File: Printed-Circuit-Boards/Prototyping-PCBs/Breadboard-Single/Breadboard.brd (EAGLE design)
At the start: 91.4 x 48.3 mm, 98 parts

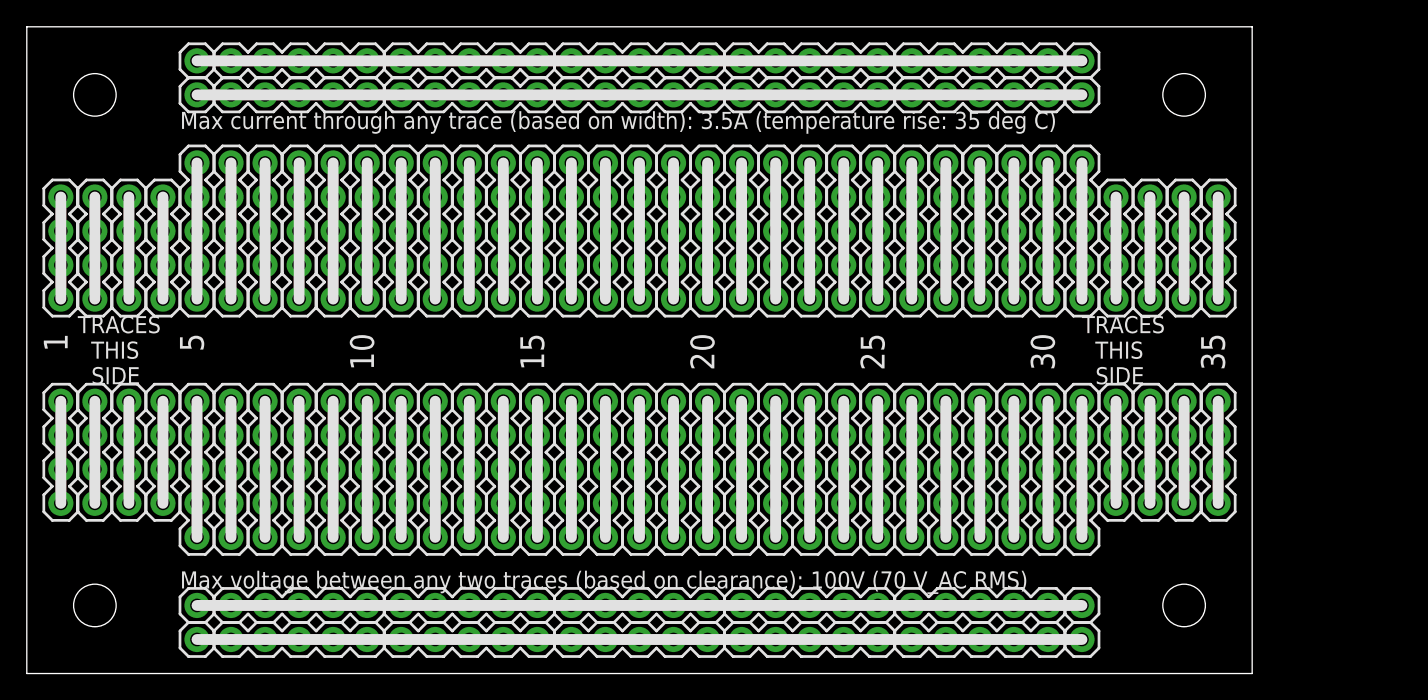
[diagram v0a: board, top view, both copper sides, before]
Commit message: Updated PCB files.
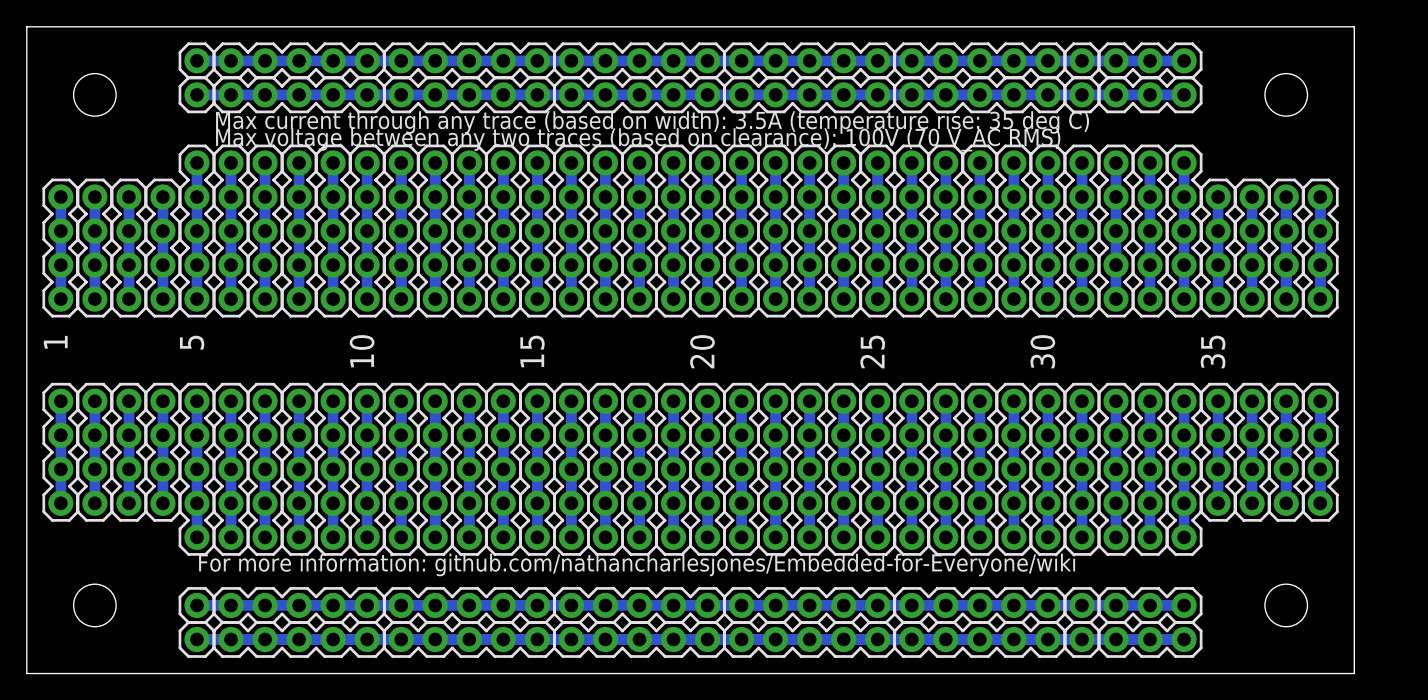
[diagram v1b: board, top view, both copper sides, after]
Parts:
- added J45, J46, J47, J48, J49, J50: (no value), SparkFun-Connectors:1X05
- added J51, J52, J53, J54: 455-1750-1-ND, SparkFun-Connectors:1X03
- moved J29 7.62 mm to (88.9, 27.9)
- moved J30 7.62 mm to (91.4, 27.9)
- moved J31 7.62 mm to (94.0, 27.9)
- moved J33 7.62 mm to (88.9, 12.7)
- moved J34 7.62 mm to (91.4, 12.7)
- moved J35 7.62 mm to (94.0, 12.7)
- moved J32 7.62 mm to (96.5, 27.9)
- moved J36 7.62 mm to (96.5, 12.7)
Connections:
- new net N$75: J48.1, J48.2, J48.3, J48.4, J48.5
- new net N$76: J45.1, J45.2, J45.3, J45.4, J45.5
- new net N$77: J46.1, J46.2, J46.3, J46.4, J46.5
- new net N$78: J47.1, J47.2, J47.3, J47.4, J47.5
- new net N$79: J49.1, J49.2, J49.3, J49.4, J49.5
- new net N$80: J50.1, J50.2, J50.3, J50.4, J50.5
- net N$1: now also J52.1, J52.2, J52.3
- net N$2: now also J51.1, J51.2, J51.3
- net N$3: now also J54.1, J54.2, J54.3
- net N$4: now also J53.1, J53.2, J53.3
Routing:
- net N$80: track 0.00 -> 10.2 mm
- net N$79: track 0.00 -> 10.2 mm
- net N$78: track 0.00 -> 10.2 mm
- net N$77: track 0.00 -> 10.2 mm
- net N$76: track 0.00 -> 10.2 mm
- net N$75: track 0.00 -> 10.2 mm
- net N$4: track 66.0 -> 73.7 mm
- net N$3: track 66.0 -> 73.7 mm
- net N$2: track 66.0 -> 73.7 mm
- net N$1: track 66.0 -> 73.7 mm
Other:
- board size 91.4 x 48.3 mm -> 99.1 x 48.3 mm
- board text added: "For more information: github.com/nathancharlesjones/Embedded-for-Everyone/wiki"
- board text removed: "For more information: nathancharlesjones@gmail.com"
